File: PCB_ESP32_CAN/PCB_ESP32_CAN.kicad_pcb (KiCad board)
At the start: 2 copper layers, 52.1 x 57.2 mm, 53 parts, among them J1 USB_C_Receptacle_USB2.0, J2 CAN, J3 CAN, J4 CAN, J5 CAN, Q1 Q_NPN_BCE, Q2 Q_NPN_BCE, U1 ESP32-WROOM-32, U2 CP2102N-A01-GQFN24, U3 SN65HVD232, U4 NCP1117-3.3_SOT223

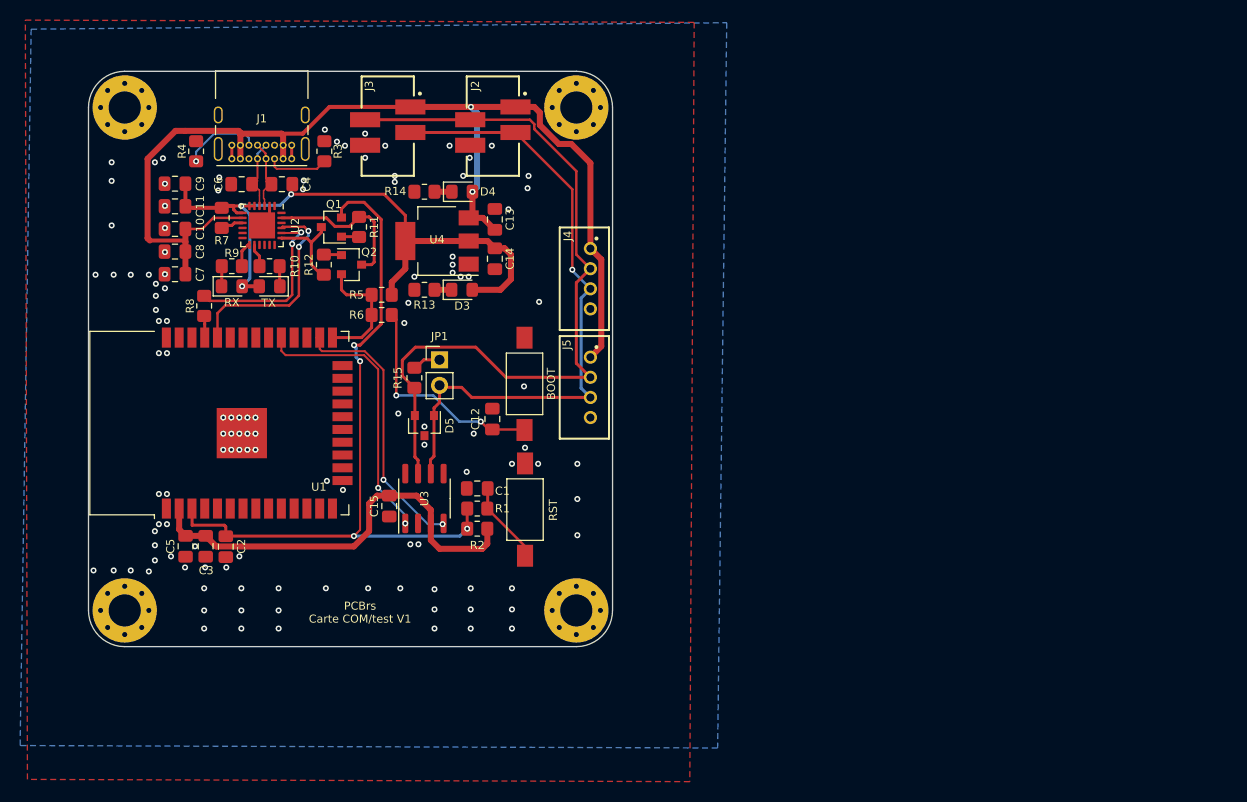
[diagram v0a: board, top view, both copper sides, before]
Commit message: V2.0 ESP32 pcb
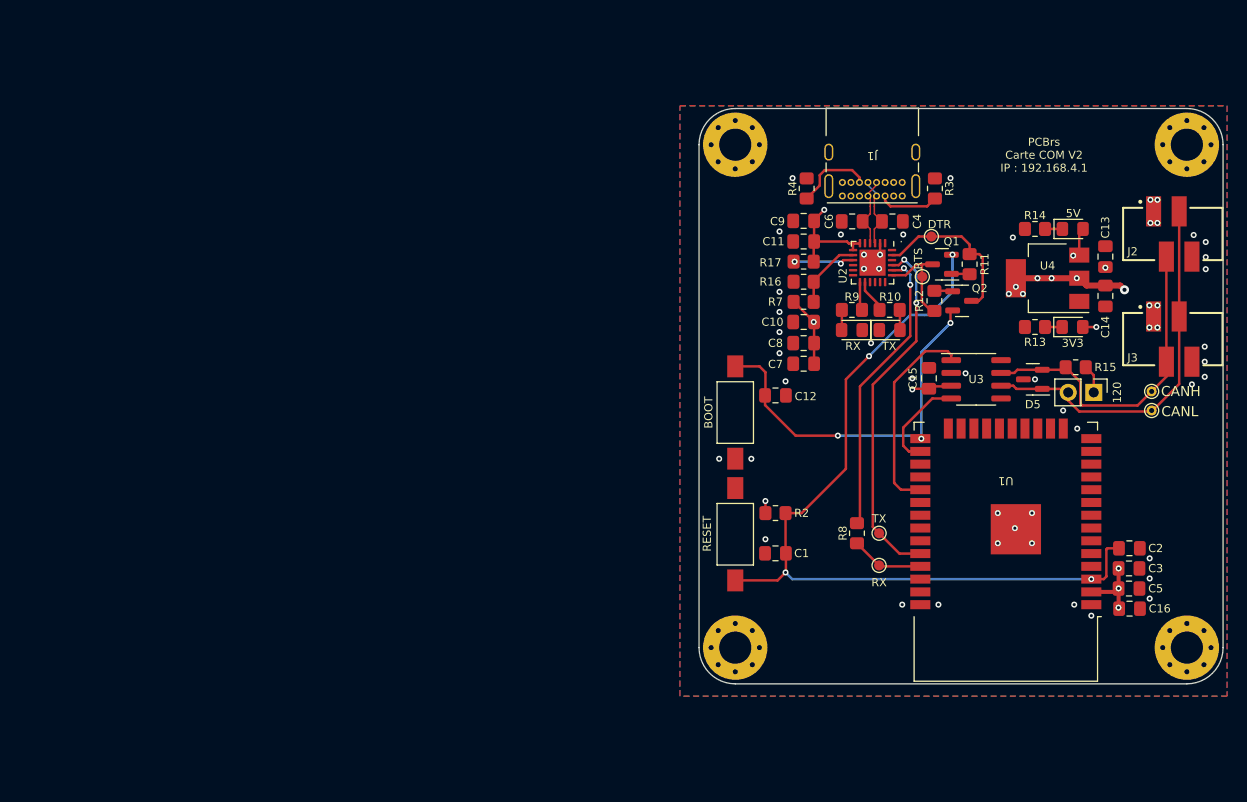
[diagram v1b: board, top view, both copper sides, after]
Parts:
- removed J4, J5: CAN, AREA_lib_Connector:Wuerth_2mm_4pin_62000411622
- removed R1, R6: 560, Resistor_SMD:R_0805_2012Metric_Pad1.20x1.40mm_HandSolder
- removed R5: 10K, Resistor_SMD:R_0805_2012Metric_Pad1.20x1.40mm_HandSolder
- added C16: 10u, Capacitor_SMD:C_0805_2012Metric_Pad1.18x1.45mm_HandSolder, F.Cu at (156.1, 123.2)
- added CANH: CANH, TestPoint:TestPoint_THTPad_D1.0mm_Drill0.5mm, F.Cu at (158.3, 101.6)
- added CANL: CANL, TestPoint:TestPoint_THTPad_D1.0mm_Drill0.5mm, F.Cu at (158.3, 103.5)
- added DTR: DTR, TestPoint:TestPoint_Pad_D1.0mm, F.Cu at (136.4, 86.2)
- added R16: 47k5, Resistor_SMD:R_0805_2012Metric_Pad1.20x1.40mm_HandSolder, F.Cu at (123.7, 90.7)
- added R17: 10k, Resistor_SMD:R_0805_2012Metric_Pad1.20x1.40mm_HandSolder, F.Cu at (123.7, 88.7)
- added RTS: RTS, TestPoint:TestPoint_Pad_D1.0mm, F.Cu at (135.5, 90.2)
- added RX: RX, TestPoint:TestPoint_Pad_D1.0mm, F.Cu at (131.2, 118.9)
- added TX: TX, TestPoint:TestPoint_Pad_D1.0mm, F.Cu at (131.2, 115.7)
- C1, C12, C2: value 1n -> 100n
- R10: value 260 -> 270
- R7: value 10K -> 22k1
- moved C5 93.9 mm to (156.1, 121.2), turned to 0 degrees
- moved C3 91.8 mm to (156.1, 119.2), turned to 0 degrees
- moved C2 89.8 mm to (156.1, 117.2), turned to 180 degrees
- moved J3 80.9 mm to (160.4, 96.4), turned to 180 degrees
- moved U1 75.8 mm to (143.8, 114.5), turned to 180 degrees
- moved R8 68.7 mm to (129.0, 115.7)
- moved J2 68.4 mm to (160.4, 86.0), turned to 180 degrees
- moved R15 65.8 mm to (150.8, 99.2), turned to 0 degrees
- moved 120 65.1 mm to (152.5, 101.7), turned to -90 degrees
- moved C10 63.2 mm to (123.7, 94.7)
- moved C8 63.2 mm to (123.7, 96.8)
- moved C7 63.1 mm to (123.7, 98.8)
- moved C9 62.6 mm to (123.7, 84.7)
- moved C11 62.6 mm to (123.7, 86.7)
- moved R10 61.8 mm to (132.2, 93.5)
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- renumbered JP1 to 120, D3 to 3V3, D4 to 5V, RST to RESET
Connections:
- BOOT pad 1: Net-(C12-Pad1) -> /IO0
- C1 pad 1: Net-(C1-Pad1) -> /EN
- C12 pad 1: Net-(C12-Pad1) -> /IO0
- J1 pad A8: Net-(J1-PadA8) -> unconnected-(J1-PadA8)
- J1 pad B8: Net-(J1-PadB8) -> unconnected-(J1-PadB8)
- R10 pad 1: Net-(D2-Pad1) -> Net-(D2-Pad2)
- R7 pad 1: +3V3 -> +5V
- R7 pad 2: Net-(R7-Pad2) -> Net-(R16-Pad1)
- R9 pad 1: Net-(D1-Pad1) -> Net-(D1-Pad2)
- RESET pad 1: Net-(C1-Pad1) -> GND
- RESET pad 2: GND -> /EN
- RX pad 1: Net-(D1-Pad1) -> GND
- RX pad 2: +3V3 -> Net-(D1-Pad2)
- TX pad 1: Net-(D2-Pad1) -> GND
- TX pad 2: +3V3 -> Net-(D2-Pad2)
- U1 pad 10: Net-(U1-Pad10) -> unconnected-(U1-Pad10)
- U1 pad 11: Net-(U1-Pad11) -> unconnected-(U1-Pad11)
- U1 pad 12: Net-(U1-Pad12) -> unconnected-(U1-Pad12)
- U1 pad 13: Net-(U1-Pad13) -> unconnected-(U1-Pad13)
- U1 pad 14: Net-(U1-Pad14) -> unconnected-(U1-Pad14)
- U1 pad 16: Net-(U1-Pad16) -> unconnected-(U1-Pad16)
- U1 pad 17: Net-(U1-Pad17) -> unconnected-(U1-Pad17)
- U1 pad 18: Net-(U1-Pad18) -> unconnected-(U1-Pad18)
- U1 pad 19: Net-(U1-Pad19) -> unconnected-(U1-Pad19)
- U1 pad 20: Net-(U1-Pad20) -> unconnected-(U1-Pad20)
- U1 pad 21: Net-(U1-Pad21) -> unconnected-(U1-Pad21)
- U1 pad 22: Net-(U1-Pad22) -> unconnected-(U1-Pad22)
- U1 pad 23: Net-(U1-Pad23) -> unconnected-(U1-Pad23)
- U1 pad 24: Net-(U1-Pad24) -> unconnected-(U1-Pad24)
- U1 pad 27: Net-(U1-Pad27) -> unconnected-(U1-Pad27)
- U1 pad 28: Net-(U1-Pad28) -> unconnected-(U1-Pad28)
- U1 pad 30: Net-(U1-Pad30) -> unconnected-(U1-Pad30)
- U1 pad 31: Net-(U1-Pad31) -> unconnected-(U1-Pad31)
- U1 pad 32: Net-(U1-Pad32) -> unconnected-(U1-Pad32)
- U1 pad 33: Net-(U1-Pad33) -> unconnected-(U1-Pad33)
- U1 pad 36: Net-(U1-Pad36) -> unconnected-(U1-Pad36)
- U1 pad 37: Net-(U1-Pad37) -> unconnected-(U1-Pad37)
- U1 pad 4: Net-(U1-Pad4) -> unconnected-(U1-Pad4)
- U1 pad 5: Net-(U1-Pad5) -> unconnected-(U1-Pad5)
- U1 pad 6: Net-(U1-Pad6) -> unconnected-(U1-Pad6)
- U1 pad 7: Net-(U1-Pad7) -> unconnected-(U1-Pad7)
- U1 pad 8: Net-(U1-Pad8) -> unconnected-(U1-Pad8)
- U1 pad 9: Net-(U1-Pad9) -> unconnected-(U1-Pad9)
- U2 pad 1: Net-(U2-Pad1) -> unconnected-(U2-Pad1)
- U2 pad 10: Net-(U2-Pad10) -> unconnected-(U2-Pad10)
- U2 pad 11: Net-(U2-Pad11) -> unconnected-(U2-Pad11)
- U2 pad 12: Net-(U2-Pad12) -> unconnected-(U2-Pad12)
- U2 pad 15: Net-(U2-Pad15) -> unconnected-(U2-Pad15)
- U2 pad 16: Net-(U2-Pad16) -> unconnected-(U2-Pad16)
- U2 pad 17: Net-(U2-Pad17) -> unconnected-(U2-Pad17)
- U2 pad 18: Net-(U2-Pad18) -> unconnected-(U2-Pad18)
- U2 pad 22: Net-(U2-Pad22) -> unconnected-(U2-Pad22)
- U2 pad 24: Net-(U2-Pad24) -> unconnected-(U2-Pad24)
- U2 pad 5: +3V3 -> unconnected-(U2-Pad5)
- U2 pad 8: +5V -> Net-(R16-Pad1)
- U2 pad 9: Net-(R7-Pad2) -> Net-(U2-Pad9)
- U3 pad 5: Net-(U3-Pad5) -> unconnected-(U3-Pad5)
- U3 pad 8: Net-(U3-Pad8) -> unconnected-(U3-Pad8)
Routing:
- net +5V: track 112.2 -> 9.81 mm, vias 2 -> 11
- net +3V3: track 108.1 -> 35.7 mm, vias 3 -> 14
- net /CANH: track 78.0 -> 32.6 mm
- net /CANL: track 65.3 -> 37.5 mm, vias 1 -> 0
- net /IO0: track 12.3 -> 37.5 mm, vias 0 -> 3
- net Net-(C12-Pad1): track 22.4 -> 0.00 mm, vias 2 -> 0
- net /RXCAN: track 27.2 -> 9.71 mm, vias 2 -> 0
- net /TX: track 21.0 -> 36.1 mm
- net Net-(R8-Pad2): track 17.8 -> 29.1 mm
- net /EN: track 71.6 -> 82.2 mm
- net Net-(C1-Pad1): track 8.26 -> 0.00 mm
- net /TXCAN: track 28.1 -> 20.5 mm, vias 2 -> 0
- net Net-(R16-Pad1): track 0.00 -> 6.97 mm
- net Net-(U2-Pad9): track 0.00 -> 6.20 mm, vias 0 -> 2
- net /RX: track 2.31 -> 7.25 mm
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- added copper zone on In1.Cu, net +3V3
- added copper zone on In1.Cu, net +5V
- added copper zone on In2.Cu, net GND
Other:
- copper layers 2 -> 4
- board text added: "."
- board text added: "PCBrs Carte COM V2 IP : 192.168.4.1"
- board text removed: "PCBrs Carte COM/test V1"
